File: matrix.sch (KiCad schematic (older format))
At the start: 89 parts

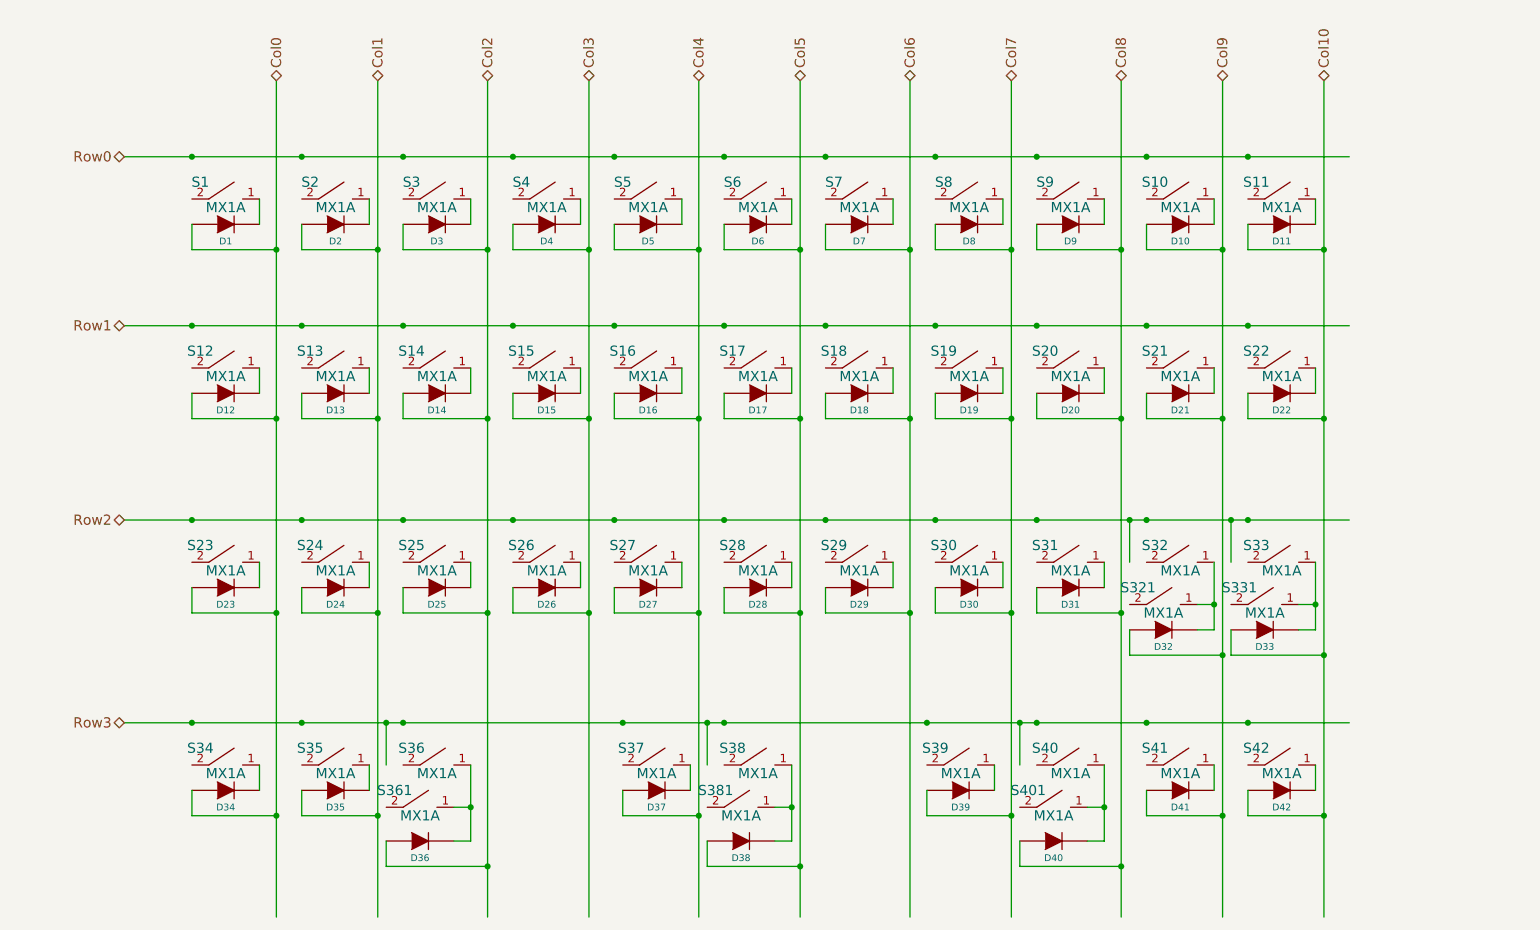
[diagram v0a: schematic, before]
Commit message: Redesign v0.3
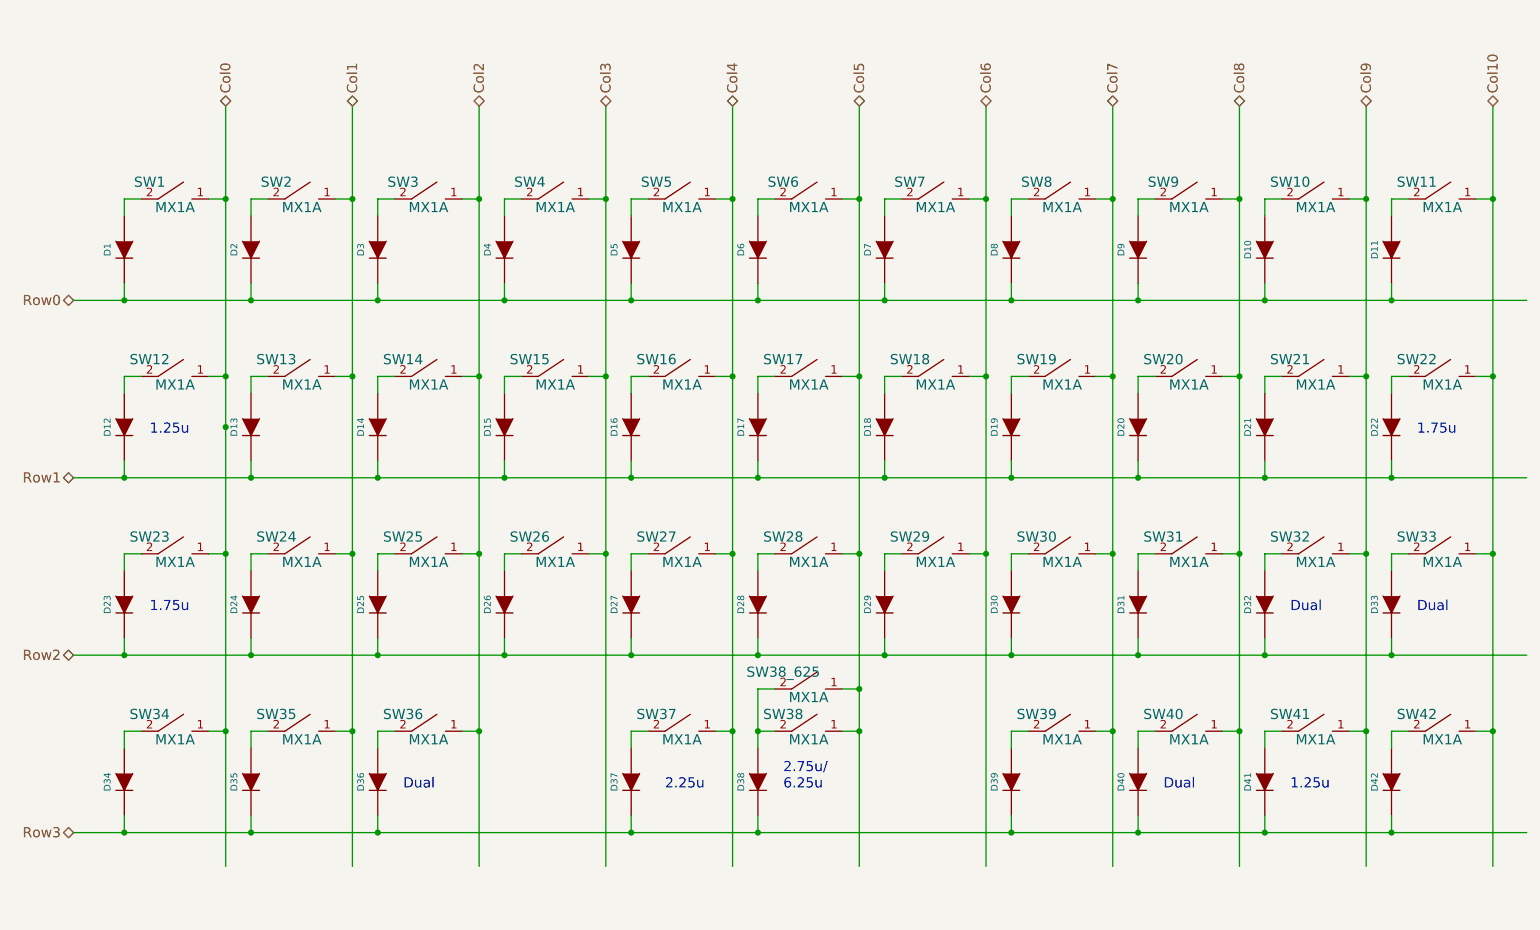
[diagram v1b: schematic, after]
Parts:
- removed S321, S331, S361, S401: MX1A, keebs:Mx_Alps_125, symbol MX1A
- D1, D10, D11, D12, D13, D14, D15, D16, D17, D18, D19, D2, D20, D21, D22, D23, D24, D25, D26, D27, D28, D29, D3, D30, D31, D32, D33, D34, D35, D36, D37, D38, D39, D4, D40, D41, D42, D5, D6, D7, D8, D9: footprint Diodes_SMD:D_SOD-123 -> diodes:D_0805_V2
- SW1: renamed from S1; footprint keebs:Mx_Alps_125 -> switches:Mx_Alps_100_NoFSilk
- SW10: renamed from S10; footprint keebs:Mx_Alps_125 -> switches:Mx_Alps_100_NoFSilk
- SW11: renamed from S11; footprint keebs:Mx_Alps_125 -> switches:Mx_Alps_100_NoFSilk
- SW12: renamed from S12; footprint keebs:Mx_Alps_125 -> switches:Mx_Alps_125_NoFSilk
- SW13: renamed from S13; footprint keebs:Mx_Alps_125 -> switches:Mx_Alps_100_NoFSilk
- SW14: renamed from S14; footprint keebs:Mx_Alps_125 -> switches:Mx_Alps_100_NoFSilk
- SW15: renamed from S15; footprint keebs:Mx_Alps_125 -> switches:Mx_Alps_100_NoFSilk
- SW16: renamed from S16; footprint keebs:Mx_Alps_125 -> switches:Mx_Alps_100_NoFSilk
- SW17: renamed from S17; footprint keebs:Mx_Alps_125 -> switches:Mx_Alps_100_NoFSilk
- SW18: renamed from S18; footprint keebs:Mx_Alps_125 -> switches:Mx_Alps_100_NoFSilk
- SW19: renamed from S19; footprint keebs:Mx_Alps_125 -> switches:Mx_Alps_100_NoFSilk
- SW2: renamed from S2; footprint keebs:Mx_Alps_125 -> switches:Mx_Alps_100_NoFSilk
- SW20: renamed from S20; footprint keebs:Mx_Alps_125 -> switches:Mx_Alps_100_NoFSilk
- SW21: renamed from S21; footprint keebs:Mx_Alps_125 -> switches:Mx_Alps_100_NoFSilk
- SW22: renamed from S22; footprint keebs:Mx_Alps_125 -> switches:Mx_Alps_175_NoFSilk
- SW23: renamed from S23; footprint keebs:Mx_Alps_125 -> switches:Mx_Alps_175_NoFSilk
- SW24: renamed from S24; footprint keebs:Mx_Alps_125 -> switches:Mx_Alps_100_NoFSilk
- SW25: renamed from S25; footprint keebs:Mx_Alps_125 -> switches:Mx_Alps_100_NoFSilk
- SW26: renamed from S26; footprint keebs:Mx_Alps_125 -> switches:Mx_Alps_100_NoFSilk
- SW27: renamed from S27; footprint keebs:Mx_Alps_125 -> switches:Mx_Alps_100_NoFSilk
- SW28: renamed from S28; footprint keebs:Mx_Alps_125 -> switches:Mx_Alps_100_NoFSilk
- SW29: renamed from S29; footprint keebs:Mx_Alps_125 -> switches:Mx_Alps_100_NoFSilk
- SW3: renamed from S3; footprint keebs:Mx_Alps_125 -> switches:Mx_Alps_100_NoFSilk
- SW30: renamed from S30; footprint keebs:Mx_Alps_125 -> switches:Mx_Alps_100_NoFSilk
- SW31: renamed from S31; footprint keebs:Mx_Alps_125 -> switches:Mx_Alps_100_NoFSilk
- SW32: renamed from S32; footprint keebs:Mx_Alps_125 -> switches:Mx_Alps_100_Dual_NoFSilk
- SW33: renamed from S33; footprint keebs:Mx_Alps_125 -> switches:Mx_Alps_100_Dual_NoFSilk
- SW34: renamed from S34; footprint keebs:Mx_Alps_125 -> switches:Mx_Alps_125_NoFSilk
- SW35: renamed from S35; footprint keebs:Mx_Alps_125 -> switches:Mx_Alps_100_NoFSilk
- SW36: renamed from S36; footprint keebs:Mx_Alps_125 -> switches:Mx_Alps_100_Dual_NoFSilk
- SW37: renamed from S37; footprint keebs:Mx_Alps_125 -> switches:Mx_Alps_225_NoFSilk
- SW38: renamed from S381; footprint keebs:Mx_Alps_125 -> switches:Mx_Alps_275_NoFSilk
- SW38_625: renamed from S38; footprint keebs:Mx_Alps_125 -> switches:Mx_Alps_625_NoFSilk
- SW39: renamed from S39; footprint keebs:Mx_Alps_125 -> switches:Mx_Alps_100_NoFSilk
- SW4: renamed from S4; footprint keebs:Mx_Alps_125 -> switches:Mx_Alps_100_NoFSilk
- SW40: renamed from S40; footprint keebs:Mx_Alps_125 -> switches:Mx_Alps_100_Dual_NoFSilk
- SW41: renamed from S41; footprint keebs:Mx_Alps_125 -> switches:Mx_Alps_125_NoFSilk
- SW42: renamed from S42; footprint keebs:Mx_Alps_125 -> switches:Mx_Alps_100_NoFSilk
- SW5: renamed from S5; footprint keebs:Mx_Alps_125 -> switches:Mx_Alps_100_NoFSilk
- SW6: renamed from S6; footprint keebs:Mx_Alps_125 -> switches:Mx_Alps_100_NoFSilk
- SW7: renamed from S7; footprint keebs:Mx_Alps_125 -> switches:Mx_Alps_100_NoFSilk
- SW8: renamed from S8; footprint keebs:Mx_Alps_125 -> switches:Mx_Alps_100_NoFSilk
- SW9: renamed from S9; footprint keebs:Mx_Alps_125 -> switches:Mx_Alps_100_NoFSilk
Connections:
- wire segments 156 -> 185
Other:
- note added: "1.25u"
- note added: "1.75u"
- note added: "2.25u"
- note added: "2.75u/\n6.25u"
- note added: "Dual"
- moved on the sheet: D1, D10, D11, D12, D13, D14, D15, D16, D17, D18, D19, D2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
